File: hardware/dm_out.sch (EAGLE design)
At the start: 42 parts, among them IC1 AOZ1280CI, IC2 ATTINY44-SSU, IC3 AOZ1280CI, Q1 BC337, Q2 BC337, X1 AKL_183-02

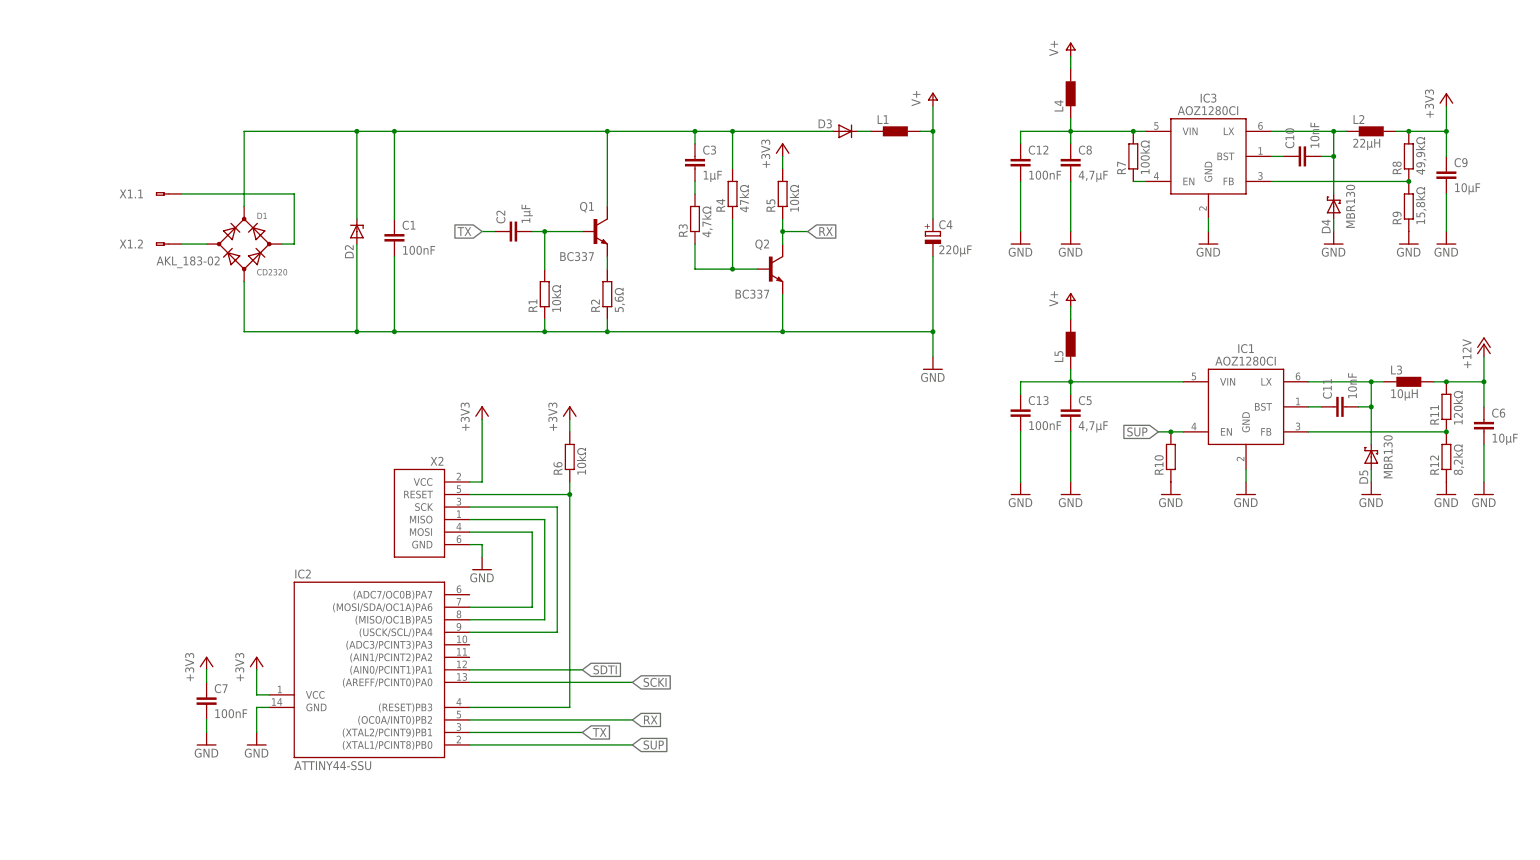
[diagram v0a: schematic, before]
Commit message: Türaußenmodul abgeschlossen
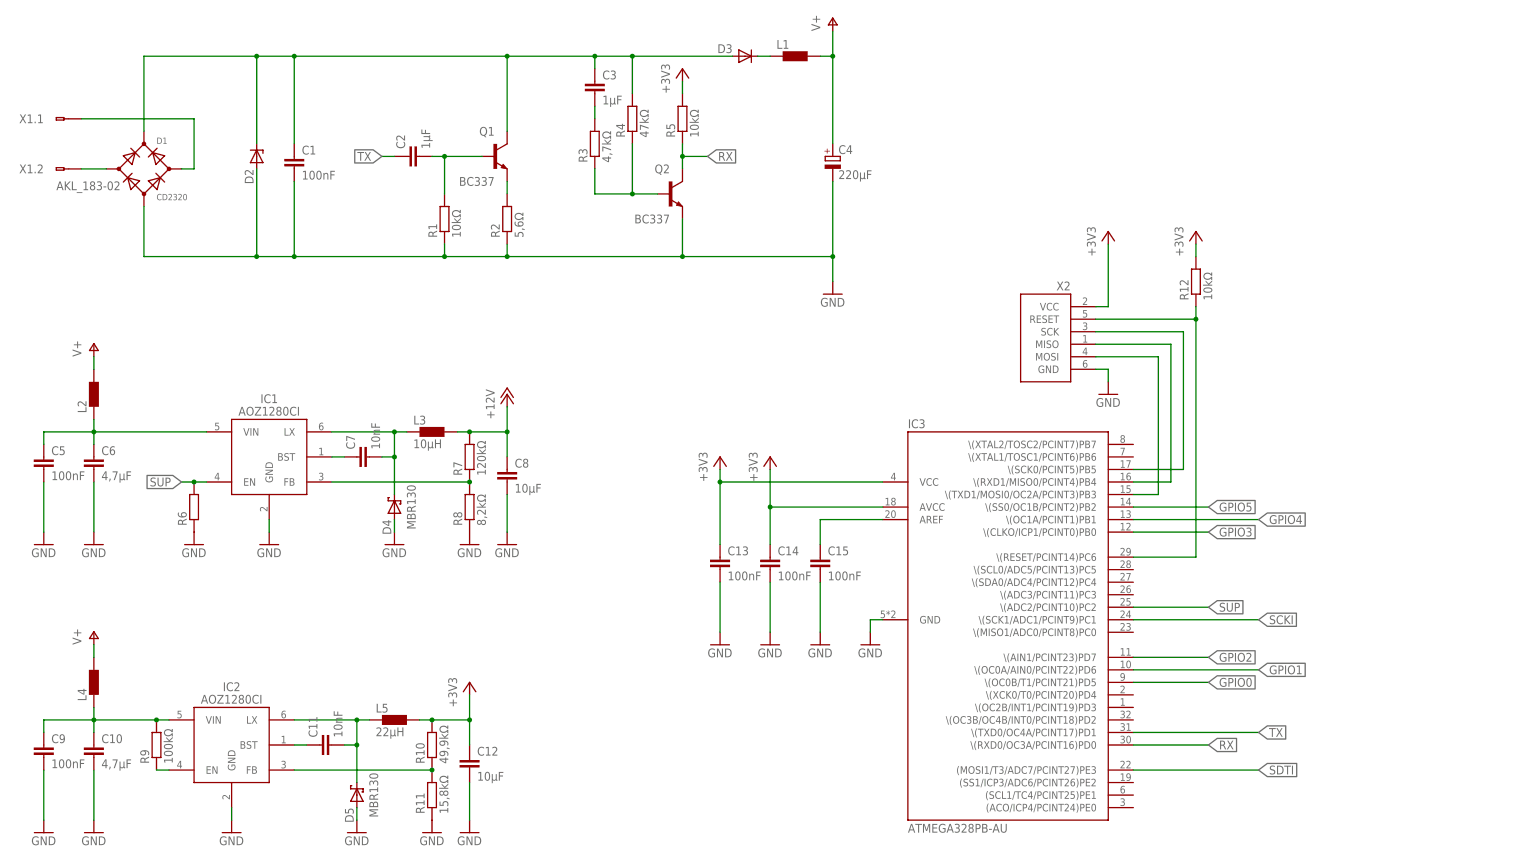
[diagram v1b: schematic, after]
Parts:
- added C14, C15: 100nF, passiv:C_0603
- C10: value 10nF -> 4,7μF; device passiv:C_0603 -> passiv:C_1206
- C12: value 100nF -> 10μF; device passiv:C_0805 -> passiv:C_1206
- C13: device passiv:C_0805 -> passiv:C_0603
- C5: value 4,7μF -> 100nF; device passiv:C_1206 -> passiv:C_0805
- C6: value 10μF -> 4,7μF
- C7: value 100nF -> 10nF
- C8: value 4,7μF -> 10μF
- C9: value 10μF -> 100nF; device passiv:C_1206 -> passiv:C_0805
- IC2: value ATTINY44-SSU -> AOZ1280CI; device ic-mcu:ATTINY44-SSU -> ic-dc_dc:AOZ1280CI
- IC3: value AOZ1280CI -> ATMEGA328PB-AU; device ic-dc_dc:AOZ1280CI -> ic-mcu:ATMEGA328PB-AU
- L2: value 22μH -> (none)
- L5: value (none) -> 22μH
- R10: value (none) -> 49,9kΩ
- R11: value 120kΩ -> 15,8kΩ
- R12: value 8,2kΩ -> 10kΩ
- R6: value 10kΩ -> (none)
- R7: value 100kΩ -> 120kΩ
- R8: value 49,9kΩ -> 8,2kΩ
- R9: value 15,8kΩ -> 100kΩ
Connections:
- new net GPIO0: IC3.\(OC0B/T1/PCINT21)PD5
- new net GPIO1: IC3.\(OC0A/AIN0/PCINT22)PD6
- new net GPIO2: IC3.\(AIN1/PCINT23)PD7
- new net GPIO3: IC3.\(CLKO/ICP1/PCINT0)PB0
- new net GPIO4: IC3.\(OC1A/PCINT1)PB1
- new net GPIO5: IC3.\(SS0/OC1B/PCINT2)PB2
- new net N$15: C15.1, IC3.AREF
- net +12V: now also C8.1, R7.2; no longer C6.1, R11.2
- net +3V3: now also C12.1, C13.1, C14.1, IC3.AVCC, IC3.VCC, L5.1, R10.2, R12.2; no longer C7.1, C9.1, IC2.VCC, L2.1, R6.2, R8.2
- net GND: now also C10.2, C14.2, C15.2, R11.1, R6.1, R8.1; no longer C7.2, R10.1, R12.1, R9.1
- net N$1: now also IC3.\(RXD1/MISO0/PCINT4)PB4; no longer IC2.(MISO/OC1B)PA5
- net N$10: now also C10.1, C9.1, IC2.VIN, R9.2; no longer C12.1, C8.1, IC3.VIN, R7.2
- net N$11: now also C7.1; no longer C11.1
- net N$12: now also C7.2, D4.K; no longer C11.2, D5.K
- net N$13: now also R7.1, R8.2; no longer R11.1, R12.2
- net N$14: now also C6.1, L2.2; no longer C13.1, L5.2
- net N$2: now also IC3.\(TXD1/MOSI0/OC2A/PCINT3)PB3; no longer IC2.(MOSI/SDA/OC1A)PA6
- net N$4: now also IC3.\(SCK0/PCINT5)PB5; no longer IC2.(USCK/SCL/)PA4
- net N$5: now also IC3.\(RESET/PCINT14)PC6, R12.1; no longer IC2.(RESET)PB3, R6.1
- net N$6: now also IC2.EN, R9.1; no longer IC3.EN, R7.1
- net N$7: now also C11.1, IC2.BST; no longer C10.1, IC3.BST
- net N$8: now also C11.2, D5.K, IC2.LX, L5.2; no longer C10.2, D4.K, IC3.LX, L2.2
- net N$9: now also IC2.FB, R10.1, R11.2; no longer IC3.FB, R8.1, R9.2
- net RX: now also IC3.\(RXD0/OC3A/PCINT16)PD0; no longer IC2.(OC0A/INT0)PB2
- net SCKI: now also IC3.\(SCK1/ADC1/PCINT9)PC1; no longer IC2.(AREFF/PCINT0)PA0
- net SDTI: now also IC3.(MOSI1/T3/ADC7/PCINT27)PE3; no longer IC2.(AIN0/PCINT1)PA1
- net SUP: now also IC3.\(ADC2/PCINT10)PC2, R6.2; no longer IC2.(XTAL1/PCINT8)PB0, R10.2
- net TX: now also IC3.\(TXD0/OC4A/PCINT17)PD1; no longer IC2.(XTAL2/PCINT9)PB1
- net V+: now also L2.1; no longer L5.1
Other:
- moved on the sheet: C1, C10, C11, C12, C13, C2, C3, C4, C5, C6, C7, C8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
